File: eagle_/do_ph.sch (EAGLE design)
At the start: 26 parts, among them IC1 MEGA8-P, Q1 8Mhz

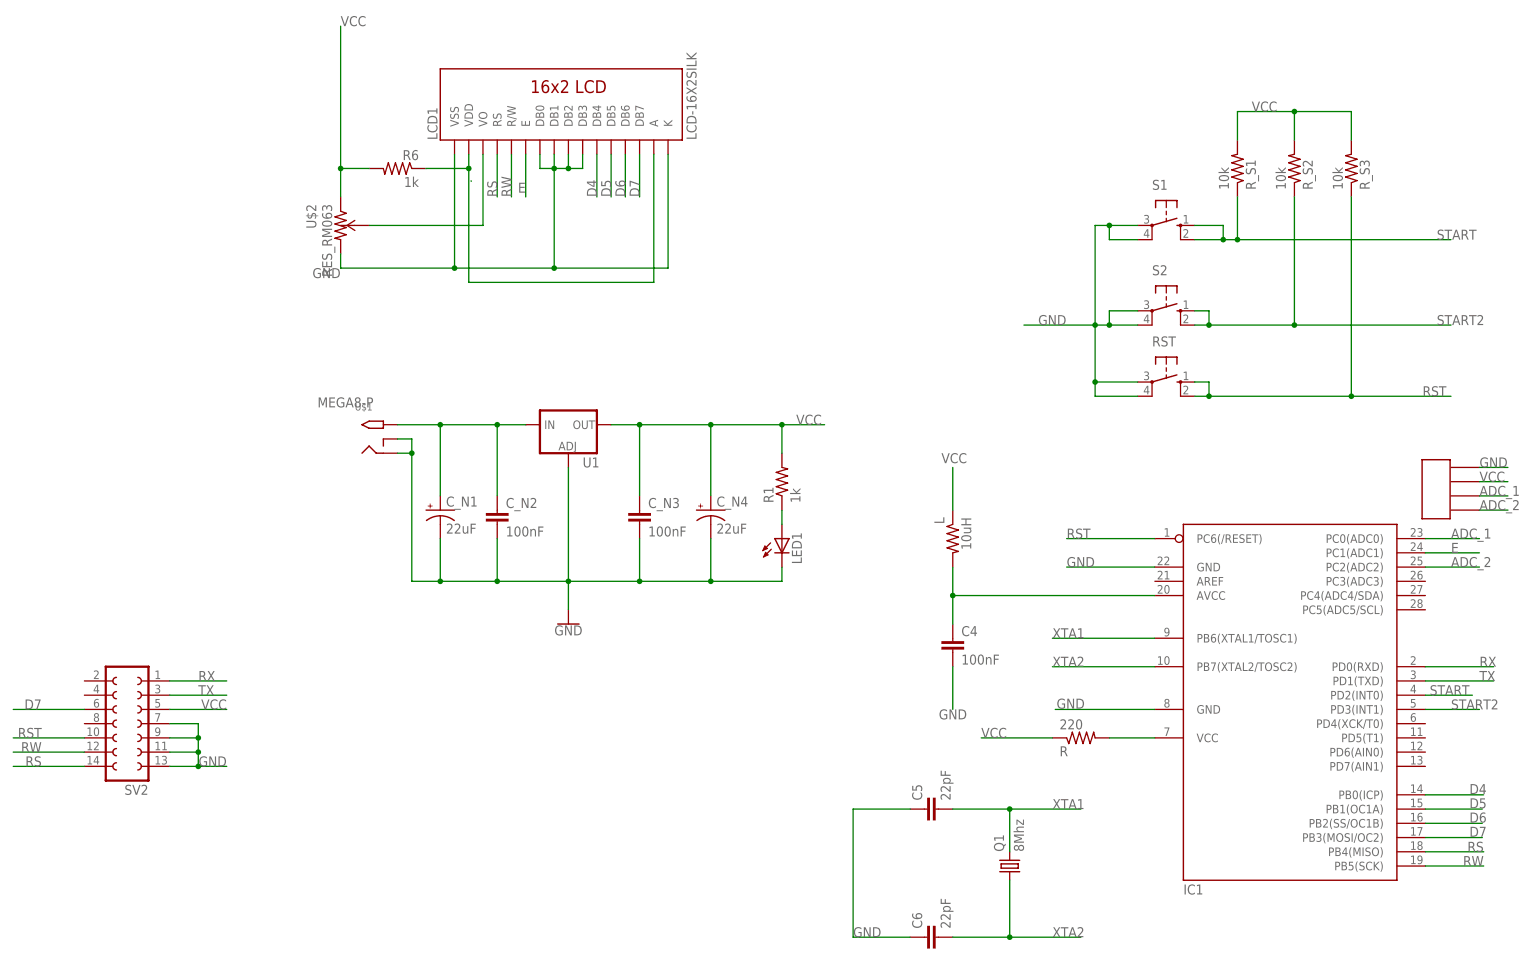
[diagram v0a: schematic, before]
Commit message: update
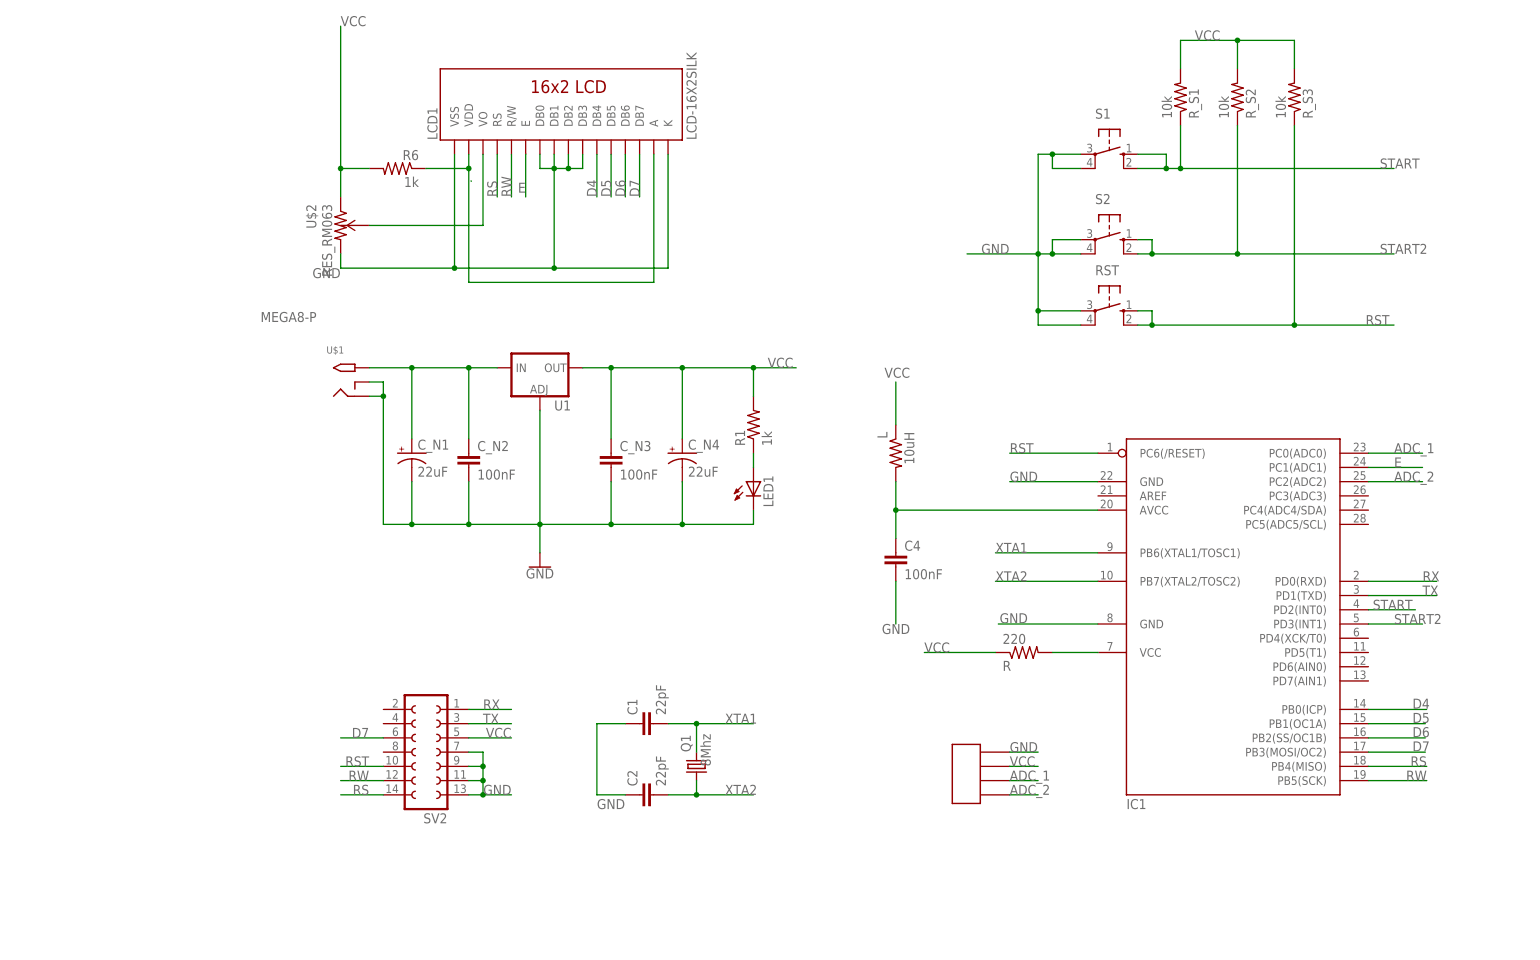
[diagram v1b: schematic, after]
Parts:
- removed C5, C6: 22pF, SparkFun-Capacitors:1.0UF-0805-25V-(+80/-20%)
- added C1, C2: 22pF, SparkFun-Retired:2.2UF-CERCAP-07888
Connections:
- net GND: now also C1.1, C2.1; no longer C5.1, C6.1
- net XTA1: now also C1.2; no longer C5.2
- net XTA2: now also C2.2; no longer C6.2
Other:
- moved on the sheet: C4, C_N1, C_N2, C_N3, C_N4, IC1, L, LED1, Q1, R, R1, RST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
